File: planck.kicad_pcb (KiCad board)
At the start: 4 copper layers, 39.4 x 58.4 mm, 53 parts, among them J1 USB_C_Receptacle_USB2.0, K1 KEYSW, K2 KEYSW, K3 KEYSW, K4 KEYSW, SW1 SW_PUSH, U1 ATmega32U4-M, Y1 Crystal_GND24_Small

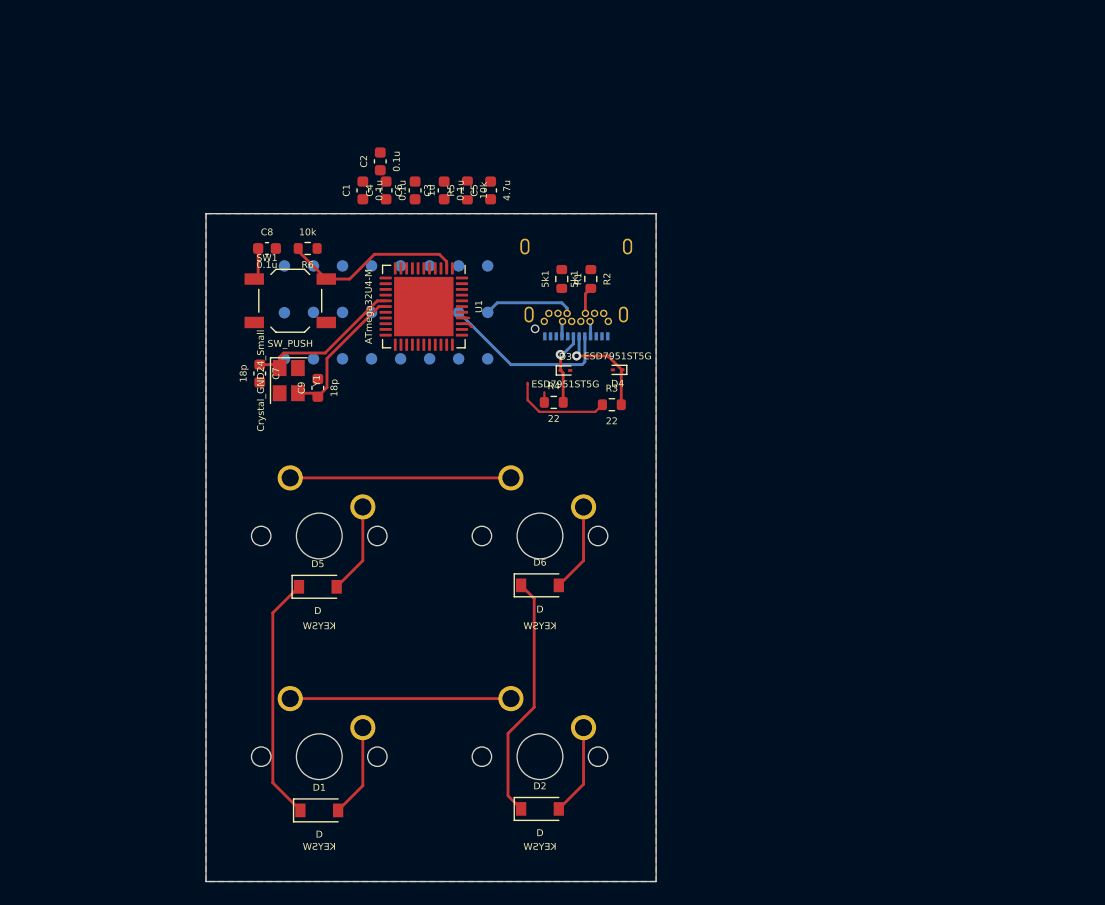
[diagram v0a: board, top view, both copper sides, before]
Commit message: finishing it off
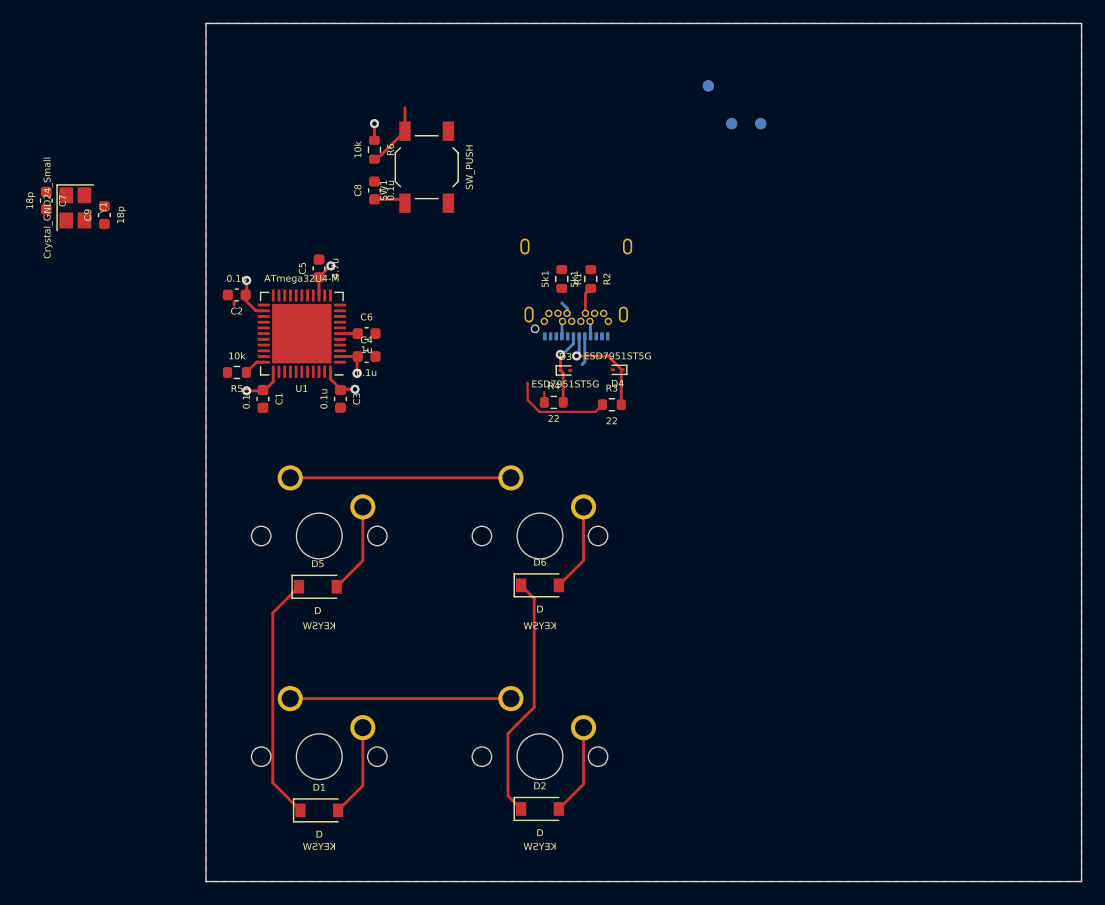
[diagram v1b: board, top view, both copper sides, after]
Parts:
- removed TP10: PB5, TestPoint:TestPoint_Pad_D1.0mm
- removed TP11: PB6, TestPoint:TestPoint_Pad_D1.0mm
- removed TP12: PB7, TestPoint:TestPoint_Pad_D1.0mm
- removed TP13: PC6, TestPoint:TestPoint_Pad_D1.0mm
- removed TP14: PC7, TestPoint:TestPoint_Pad_D1.0mm
- removed TP15: PD0, TestPoint:TestPoint_Pad_D1.0mm
- removed TP16: PD1, TestPoint:TestPoint_Pad_D1.0mm
- removed TP17: PD2, TestPoint:TestPoint_Pad_D1.0mm
- removed TP18: PD3, TestPoint:TestPoint_Pad_D1.0mm
- removed TP19: PD4, TestPoint:TestPoint_Pad_D1.0mm
- removed TP20: PD6, TestPoint:TestPoint_Pad_D1.0mm
- removed TP21: PD7, TestPoint:TestPoint_Pad_D1.0mm
- removed TP22: PE6, TestPoint:TestPoint_Pad_D1.0mm
- removed TP23: PF6, TestPoint:TestPoint_Pad_D1.0mm
- removed TP24: PF7, TestPoint:TestPoint_Pad_D1.0mm
- removed TP4: PD5, TestPoint:TestPoint_Pad_D1.0mm
- removed TP5: PB0, TestPoint:TestPoint_Pad_D1.0mm
- removed TP6: PB1, TestPoint:TestPoint_Pad_D1.0mm
- removed TP7: PB2, TestPoint:TestPoint_Pad_D1.0mm
- removed TP8: PB3, TestPoint:TestPoint_Pad_D1.0mm
- removed TP9: PB4, TestPoint:TestPoint_Pad_D1.0mm
- moved TP3 31.4 mm to (121.4, 67.6)
- moved TP1 29.0 mm to (123.4, 70.9)
- moved TP2 29.0 mm to (126.0, 70.9)
- moved R5 25.7 mm to (80.2, 92.6), turned to 180 degrees
- moved C7 24.0 mm to (63.5, 77.6)
- moved C9 24.0 mm to (68.6, 78.9)
- moved Y1 24.0 mm to (66.0, 78.2)
- moved C3 20.4 mm to (89.2, 94.9), turned to -90 degrees
- moved C1 20.2 mm to (82.4, 94.9), turned to -90 degrees
- moved C2 17.1 mm to (80.2, 85.9), turned to 180 degrees
- moved SW1 16.7 mm to (96.8, 74.7), turned to 90 degrees
- moved C5 16.5 mm to (87.3, 83.5)
- moved C4 14.6 mm to (91.5, 91.2), turned to 0 degrees
- moved C6 13.2 mm to (91.5, 89.2), turned to 0 degrees
- moved U1 10.9 mm to (85.8, 89.2), turned to 180 degrees
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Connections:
- U1 pad 1: /PE6 -> unconnected-(U1-Pad1)
- U1 pad 10: /PB2 -> unconnected-(U1-Pad10)
- U1 pad 11: /PB3 -> unconnected-(U1-Pad11)
- U1 pad 12: /PB7 -> unconnected-(U1-Pad12)
- U1 pad 18: /PD0 -> unconnected-(U1-Pad18)
- U1 pad 19: /PD1 -> unconnected-(U1-Pad19)
- U1 pad 20: /PD2 -> unconnected-(U1-Pad20)
- U1 pad 21: /PD3 -> unconnected-(U1-Pad21)
- U1 pad 22: /PD5 -> unconnected-(U1-Pad22)
- U1 pad 25: /PD4 -> unconnected-(U1-Pad25)
- U1 pad 26: /PD6 -> unconnected-(U1-Pad26)
- U1 pad 27: /PD7 -> unconnected-(U1-Pad27)
- U1 pad 28: /PB4 -> unconnected-(U1-Pad28)
- U1 pad 29: /PB5 -> unconnected-(U1-Pad29)
- U1 pad 30: /PB6 -> unconnected-(U1-Pad30)
- U1 pad 31: /PC6 -> unconnected-(U1-Pad31)
- U1 pad 32: /PC7 -> unconnected-(U1-Pad32)
- U1 pad 36: /PF7 -> unconnected-(U1-Pad36)
- U1 pad 37: /PF6 -> unconnected-(U1-Pad37)
- U1 pad 8: /PB0 -> unconnected-(U1-Pad8)
- U1 pad 9: /PB1 -> unconnected-(U1-Pad9)
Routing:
- net VCC: track 2.66 -> 20.7 mm, vias 0 -> 6
- net /XTAL2: track 14.2 -> 0.00 mm
- net Net-(J1-PadA8): track 15.3 -> 2.57 mm
- net /XTAL1: track 12.6 -> 0.00 mm
- net /~reset: track 18.8 -> 7.85 mm
- net Net-(J1-PadB8): track 7.95 -> 1.12 mm
- net Net-(R5-Pad1): track 0.00 -> 1.89 mm
- net Net-(C6-Pad1): track 0.00 -> 1.56 mm
- net /PF7: track 0.97 -> 0.00 mm
- net /PF6: track 0.63 -> 0.00 mm
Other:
- board size 39.4 x 58.4 mm -> 76.6 x 75.1 mm
